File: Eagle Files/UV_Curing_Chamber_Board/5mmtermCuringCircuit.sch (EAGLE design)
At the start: 25 parts, among them IC1 7805T, IC2 L293D, T1 RFP30N06LE, T2 RFP30N06LE

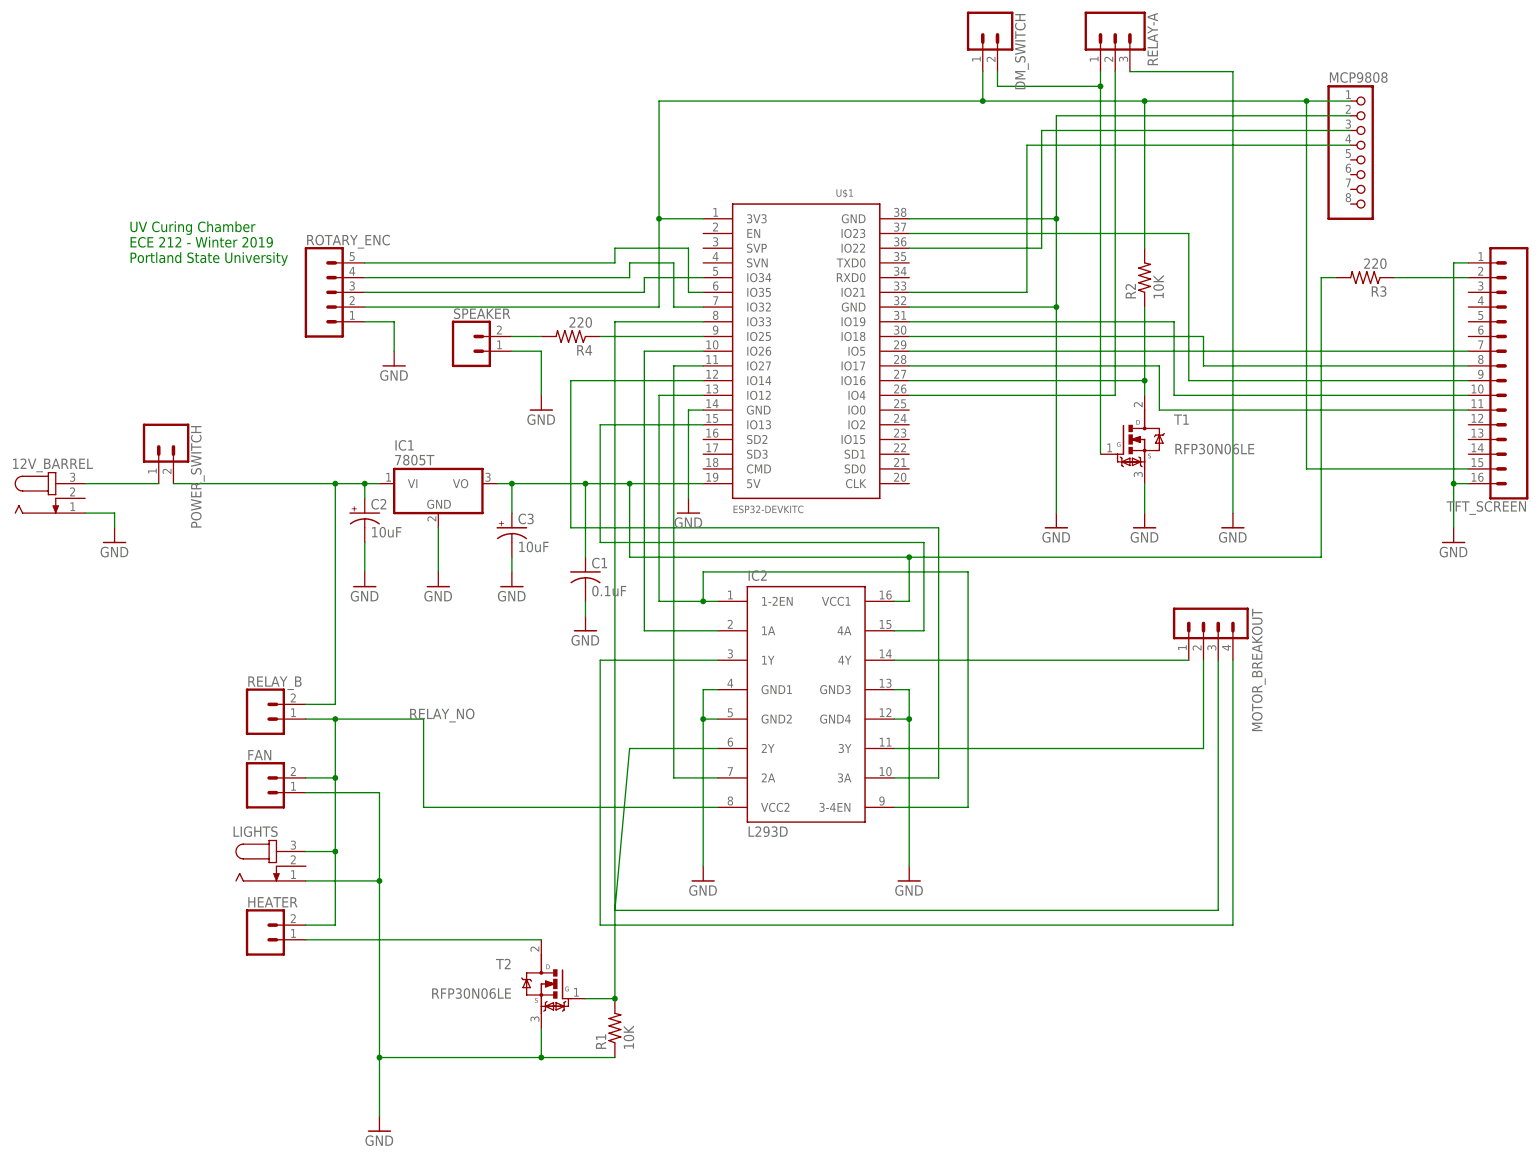
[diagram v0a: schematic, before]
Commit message: more eagle
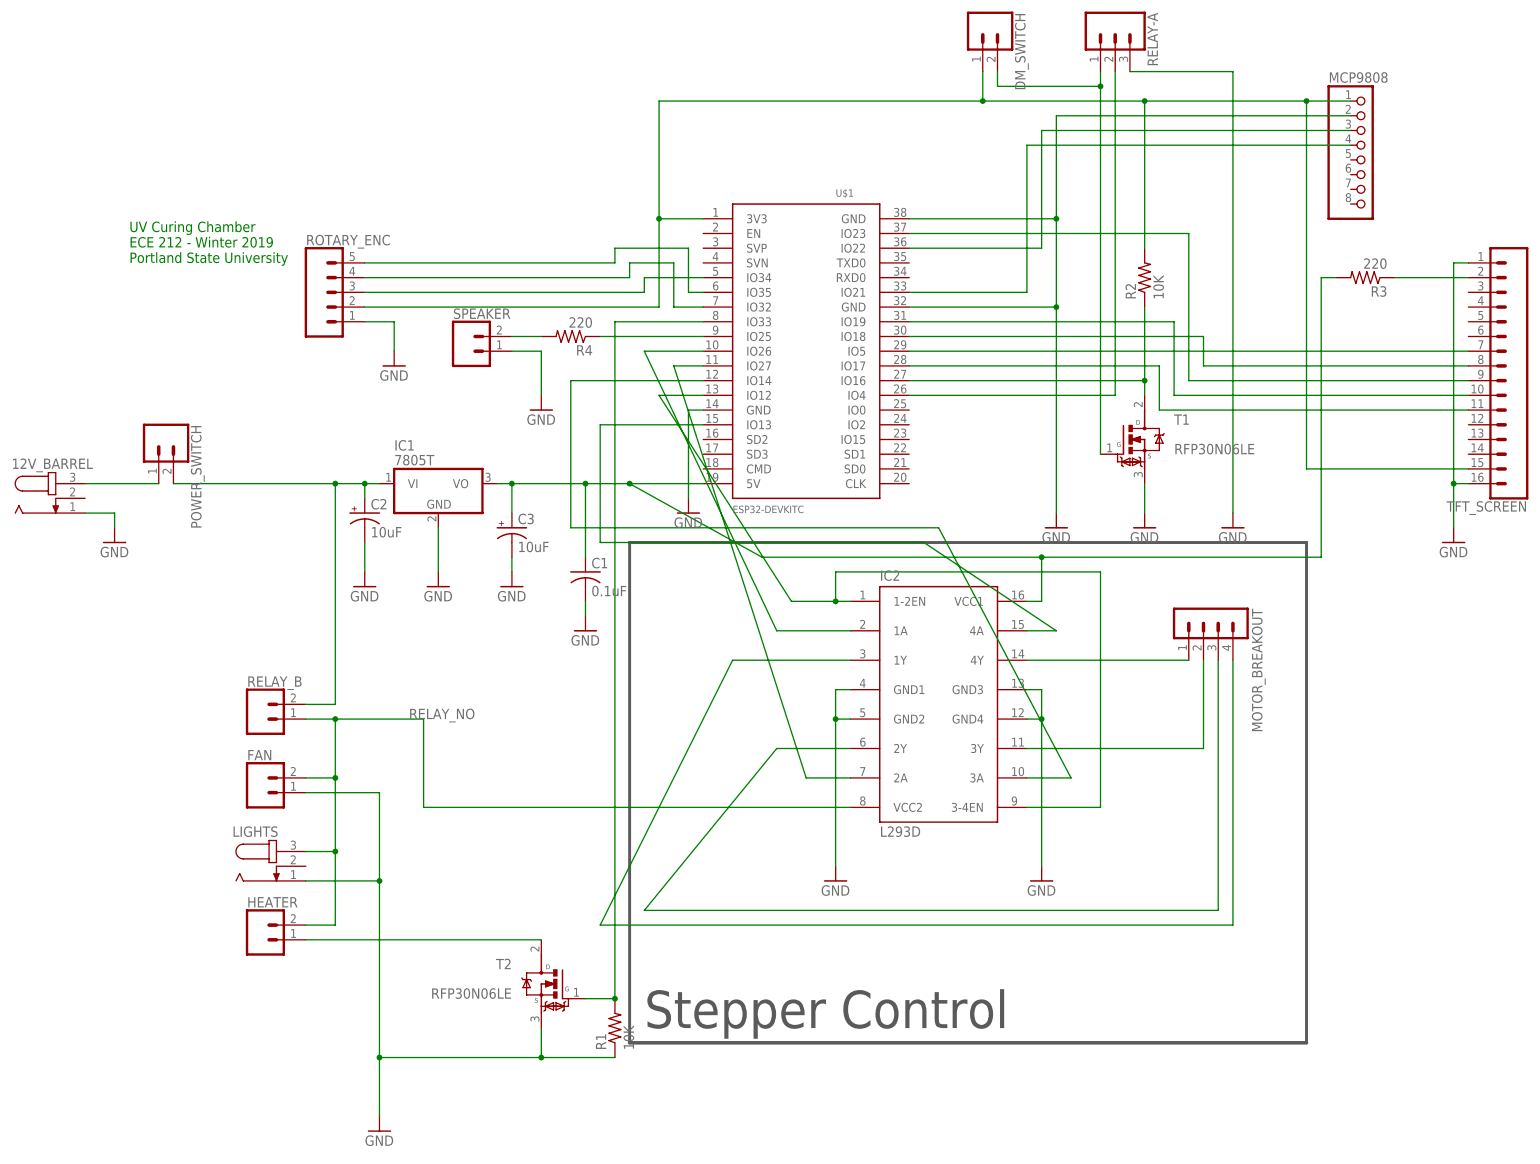
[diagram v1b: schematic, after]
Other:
- note added: "Stepper Control"
- moved on the sheet: IC2

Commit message: schematic
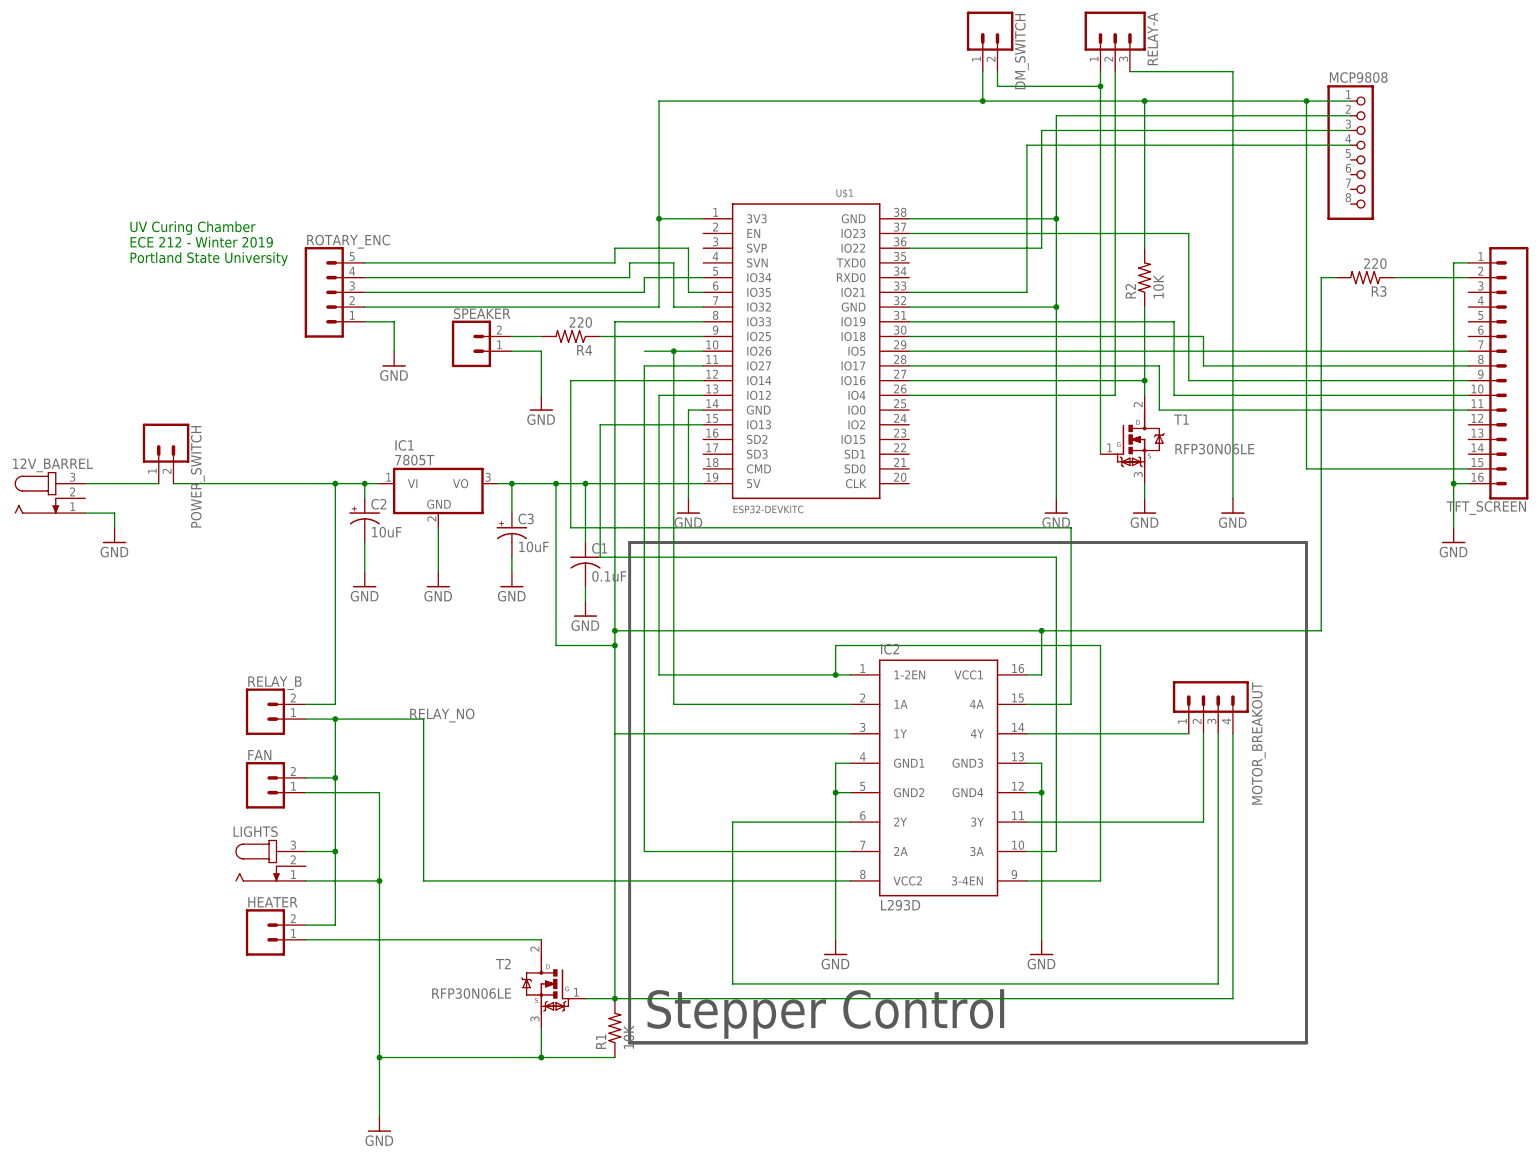
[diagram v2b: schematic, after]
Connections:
- removed net N$1: C1.1, C3.+, IC1.VO, IC2.VCC1, R3.2, U$1.5V
- removed net N$30: IC2.3A, U$1.IO14
- removed net N$5 (its old number): R1.2, T2.G, U$1.IO33
- new net N$2: IC2.4A, U$1.IO14
- net N$14: now also C1.1, C3.+, IC1.VO, IC2.VCC1, R1.2, R3.2, T2.G, U$1.5V, U$1.IO33
- net N$29: now also IC2.3A; no longer IC2.4A
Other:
- moved on the sheet: C1, IC2, MOTOR_BREAKOUT
